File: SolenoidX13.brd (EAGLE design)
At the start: 35.6 x 30.5 mm, 24 parts, among them J1 SAMTEC-CLT-111-01-X-DJ, U1 ULN2003V12

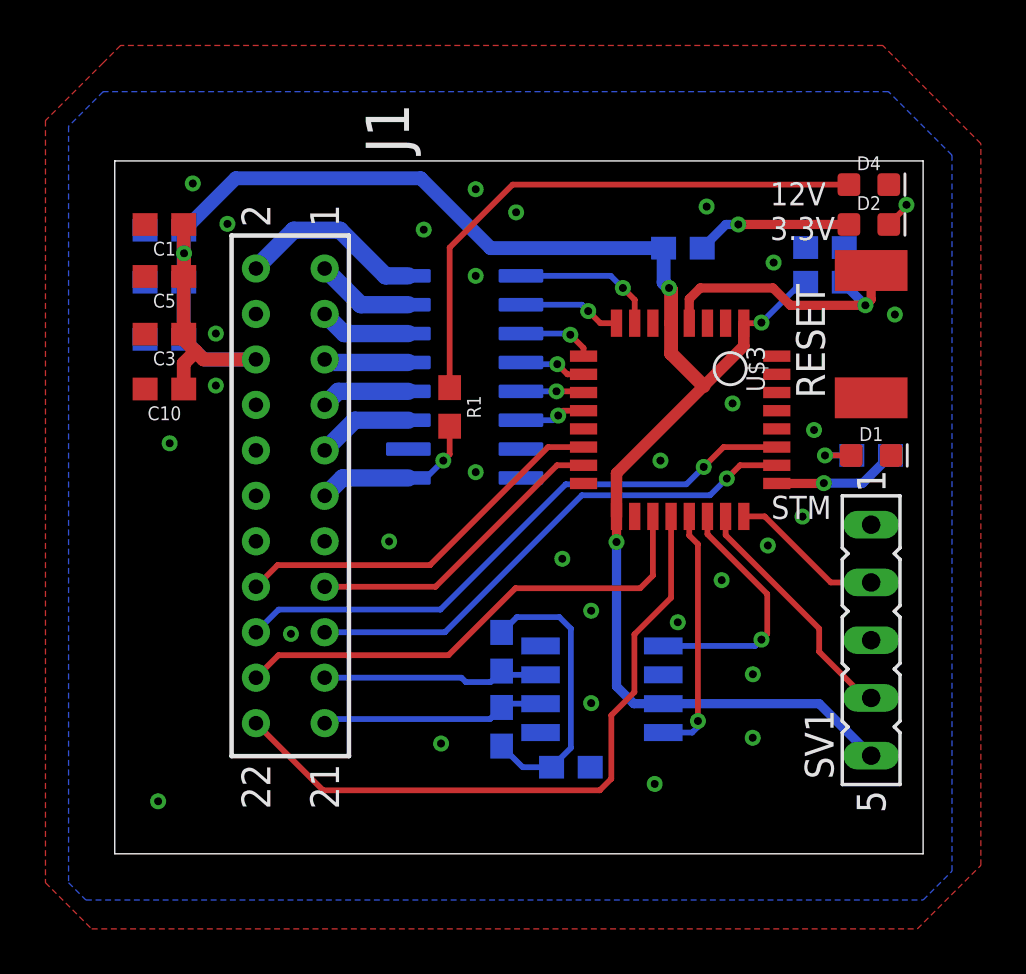
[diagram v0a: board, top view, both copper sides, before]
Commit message: lol
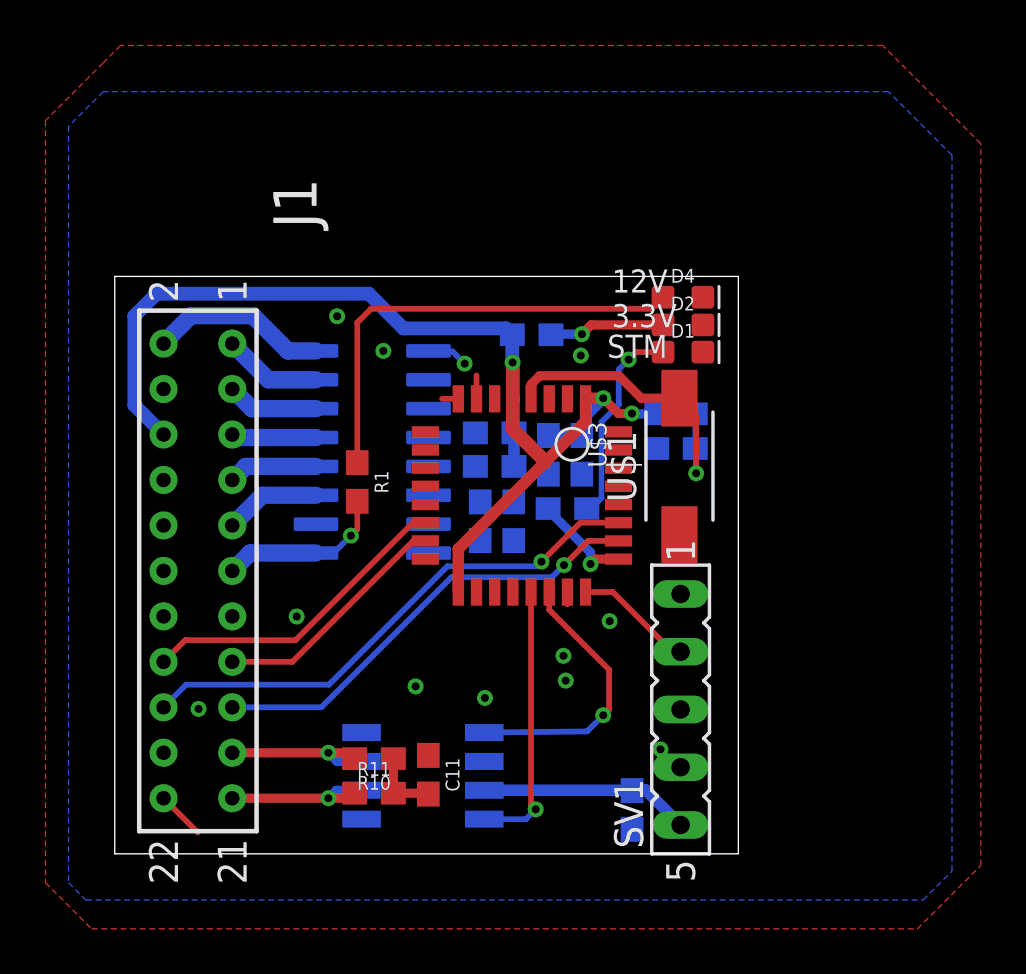
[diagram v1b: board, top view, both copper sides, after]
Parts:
- removed RESET: (no value), DiscreteComponents:SW_2512
- added U$1: (no value), Push button - FSM2JMTR:DISCRETECOMPONENTS_SW_2512
- moved C10 27.7 mm to (22.8, 1.93), flipped to the bottom, turned to 270 degrees
- moved C4 20.0 mm to (17.6, 14.6), turned to 90 degrees
- moved C1 19.7 mm to (19.1, 17.6), flipped to the bottom, turned to 270 degrees
- moved C3 19.1 mm to (20.5, 17.6), flipped to the bottom, turned to 270 degrees
- moved C5 16.8 mm to (16.7, 17.0), flipped to the bottom, turned to 0 degrees
- moved C2 16.0 mm to (16.1, 14.6), turned to 90 degrees
- moved C6 16.0 mm to (16.7, 18.5)
- moved R7 13.6 mm to (19.9, 15.2), turned to 0 degrees
- moved C7 11.0 mm to (24.7, 17.8)
- moved D4 9.56 mm to (25.0, 24.5)
- moved D1 9.45 mm to (25.0, 22.1)
- moved D2 9.30 mm to (25.0, 23.3)
- moved SV1 8.92 mm to (24.9, 6.35)
- moved U$8 8.75 mm to (16.3, 1.52)
- moved R2 8.75 mm to (24.7, 19.4)
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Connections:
- net GND: now also U$1.1; no longer RESET.1
- net NRST1: now also U$1.2; no longer RESET.2
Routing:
- net DATA: track 29.7 -> 2.13 mm
- net CLK: track 21.9 -> 0.00 mm
- net +3V3: track 83.2 -> 61.9 mm, vias 4 -> 3
- net SWCLK: track 10.8 -> 0.54 mm
- net N$5: track 12.6 -> 3.08 mm
- net N$24: track 2.34 -> 9.08 mm
- net N$25: track 24.9 -> 20.1 mm
- net GPIO1: track 6.47 -> 2.84 mm
- net GPIO2: track 4.54 -> 0.95 mm, vias 1 -> 0
- net GPIO3: track 3.38 -> 0.00 mm, vias 1 -> 0
- net GPIO4: track 2.97 -> 0.00 mm, vias 1 -> 0
- net GPIO6: track 2.93 -> 0.00 mm, vias 1 -> 0
- net ALERT1: track 26.3 -> 23.4 mm
- net C2_1: track 17.0 -> 14.1 mm
- net C2_2: track 13.6 -> 10.7 mm
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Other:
- board size 35.6 x 30.5 mm -> 27.4 x 25.4 mm
